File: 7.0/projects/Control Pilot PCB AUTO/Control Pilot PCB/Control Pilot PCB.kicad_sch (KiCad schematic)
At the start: 25 parts, among them J1 Conn_01x01, J2 Conn_01x01, J3 Conn_01x01, J4 Conn_01x01, J5 Conn_01x01, Q1 AO3400A, Q2 AO3400A, SW1 SW_SPDT, SW2 SW_SPDT, SW3 SW_SPDT, SW5 SW_SPDT, SW6 SW_SPDT, SW7 SW_SPDT

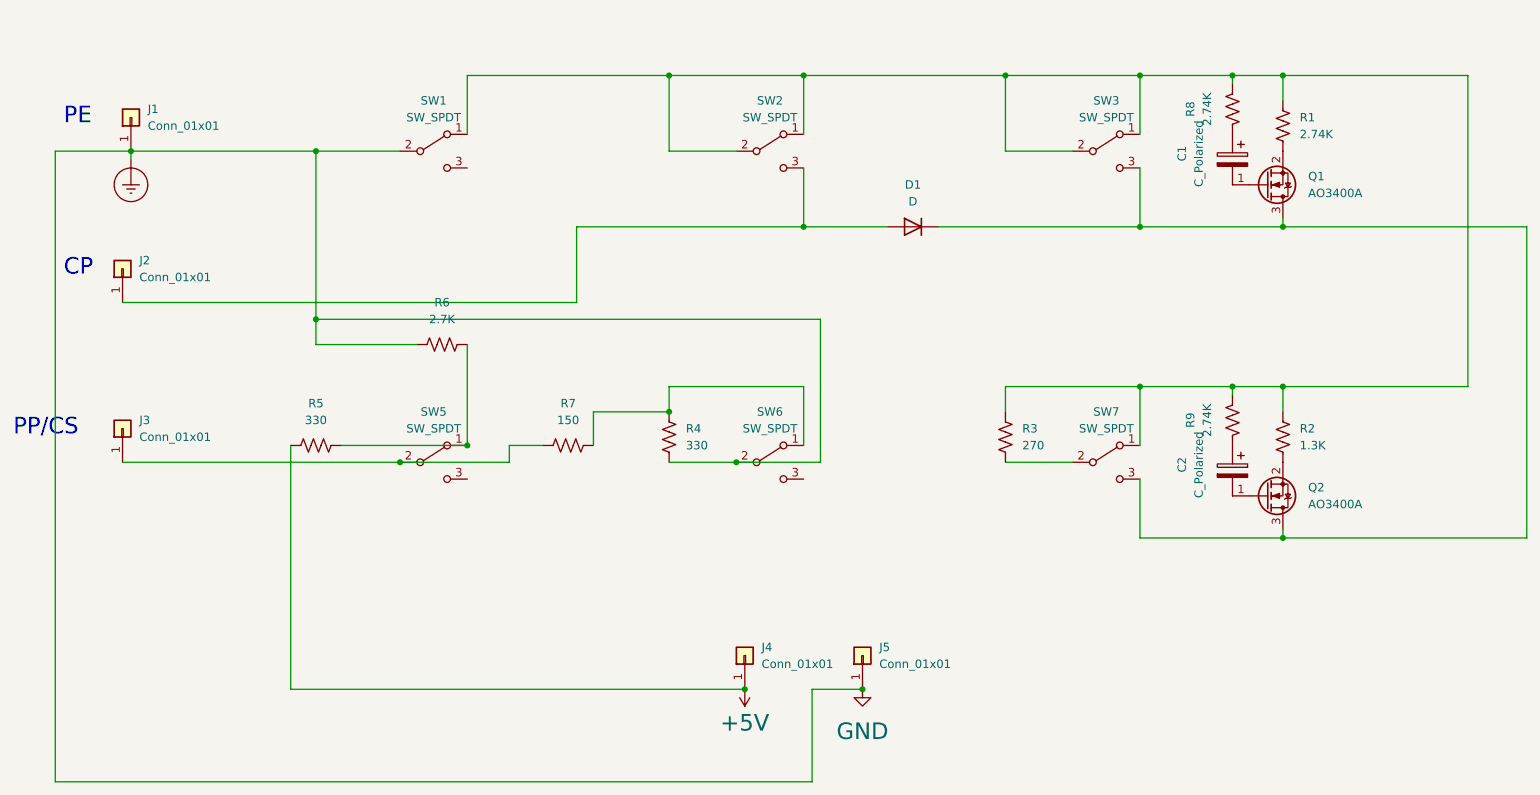
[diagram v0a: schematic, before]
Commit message: Update
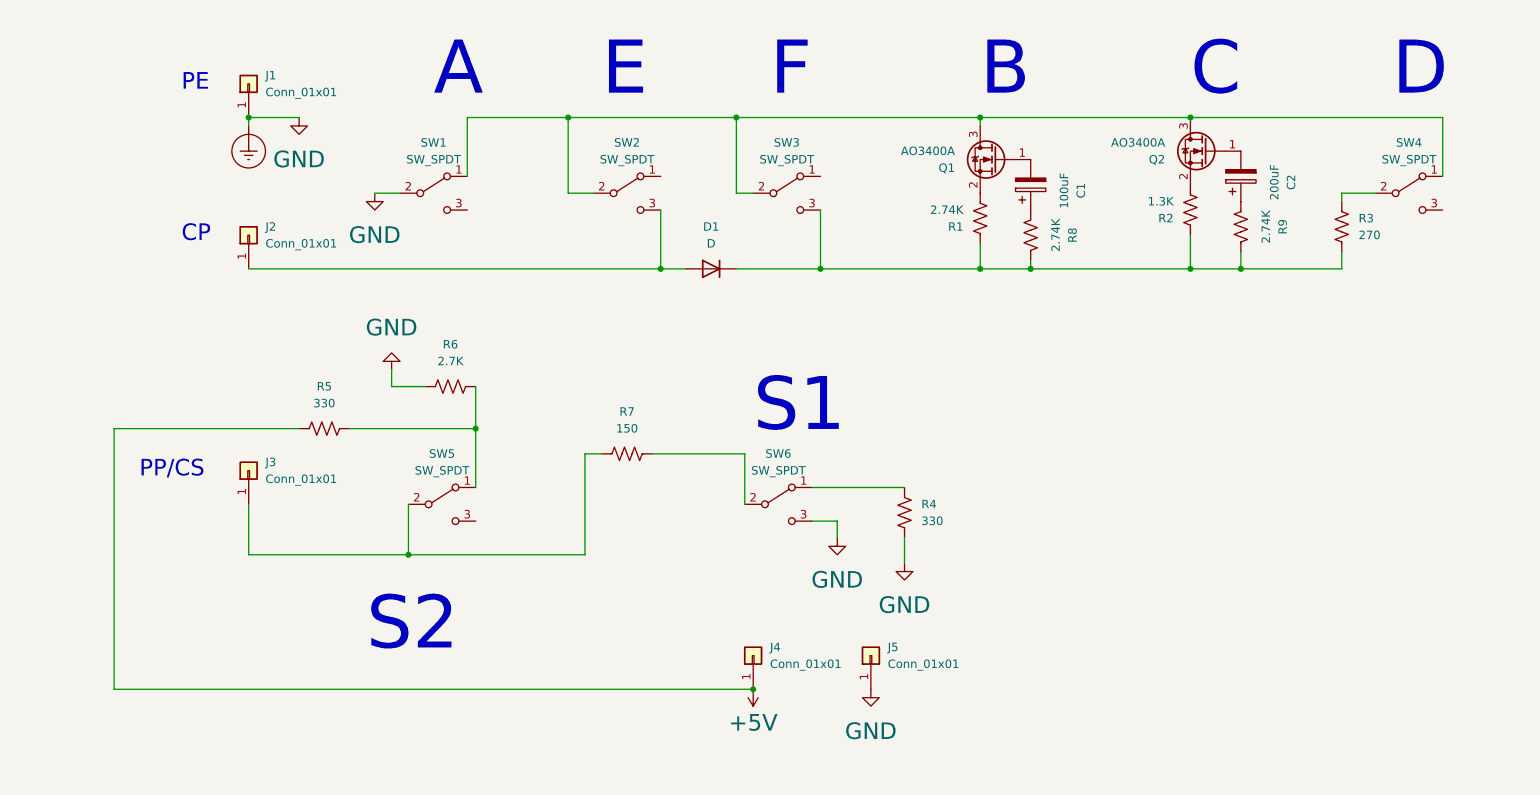
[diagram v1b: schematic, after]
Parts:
- removed SW7: SW_SPDT, Connector_PinHeader_2.54mm:PinHeader_1x03_P2.54mm_Vertical, symbol Switch:SW_SPDT
- added SW4: SW_SPDT, Connector_PinHeader_2.54mm:PinHeader_1x03_P2.54mm_Vertical, symbol Switch:SW_SPDT
- C1: value C_Polarized -> 100uF
- C2: value C_Polarized -> 200uF
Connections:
- net Earth_Protective: now also SW6.3 (C); no longer SW6.2 (B)
- net at Q1.3 (D), Q2.3 (D): now also SW1.1 (A), SW2.2 (B), SW3.2 (B), SW4.1 (A); no longer D1.1 (K), SW3.3 (C)
- net at R4.1, SW6.1 (A): no longer R7.1
- net at R3.2: now also D1.1 (K), R1.1, R2.1, R8.1, R9.1, SW3.3 (C)
- new net: R7.1, SW6.2 (B)
- new net: R3.1, SW4.2 (B)
- now unconnected: SW2.1 (A), SW3.1 (A)
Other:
- note added: "A"
- note added: "B"
- note added: "C"
- note added: "D"
- note added: "E"
- note added: "F"
- note added: "S1"
- note added: "S2"
- moved on the sheet: C1, D1, J1, J2, J3, J4, J5, Q1, R1, R5, R6, R8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
